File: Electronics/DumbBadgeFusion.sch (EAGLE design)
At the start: 103 parts, among them IC1 SN74CBT16233DGGR, IC2 SN74CBT16233DGGR, SW1 SPST_TACT-KMR2, U1 TDP3E001DRLR-SOT-23-5SOT-23-5, U6 MAX3232, U7 TPS61090RSAR, U8 MCP73831T-2ACI/OT, X4 32.768

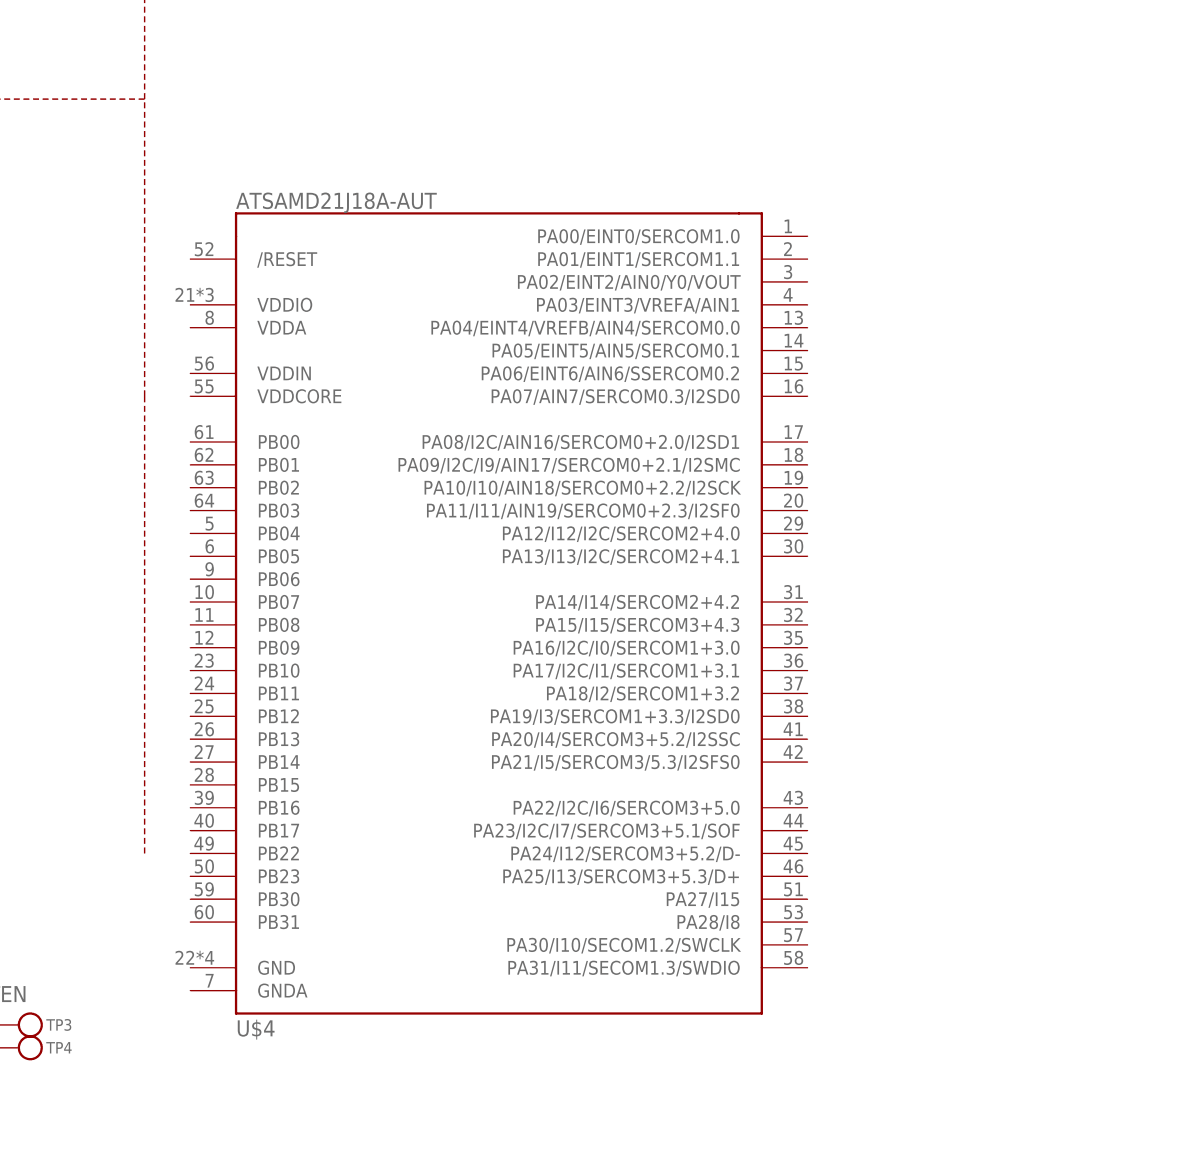
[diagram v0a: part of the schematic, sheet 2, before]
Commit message: beginning Firmware
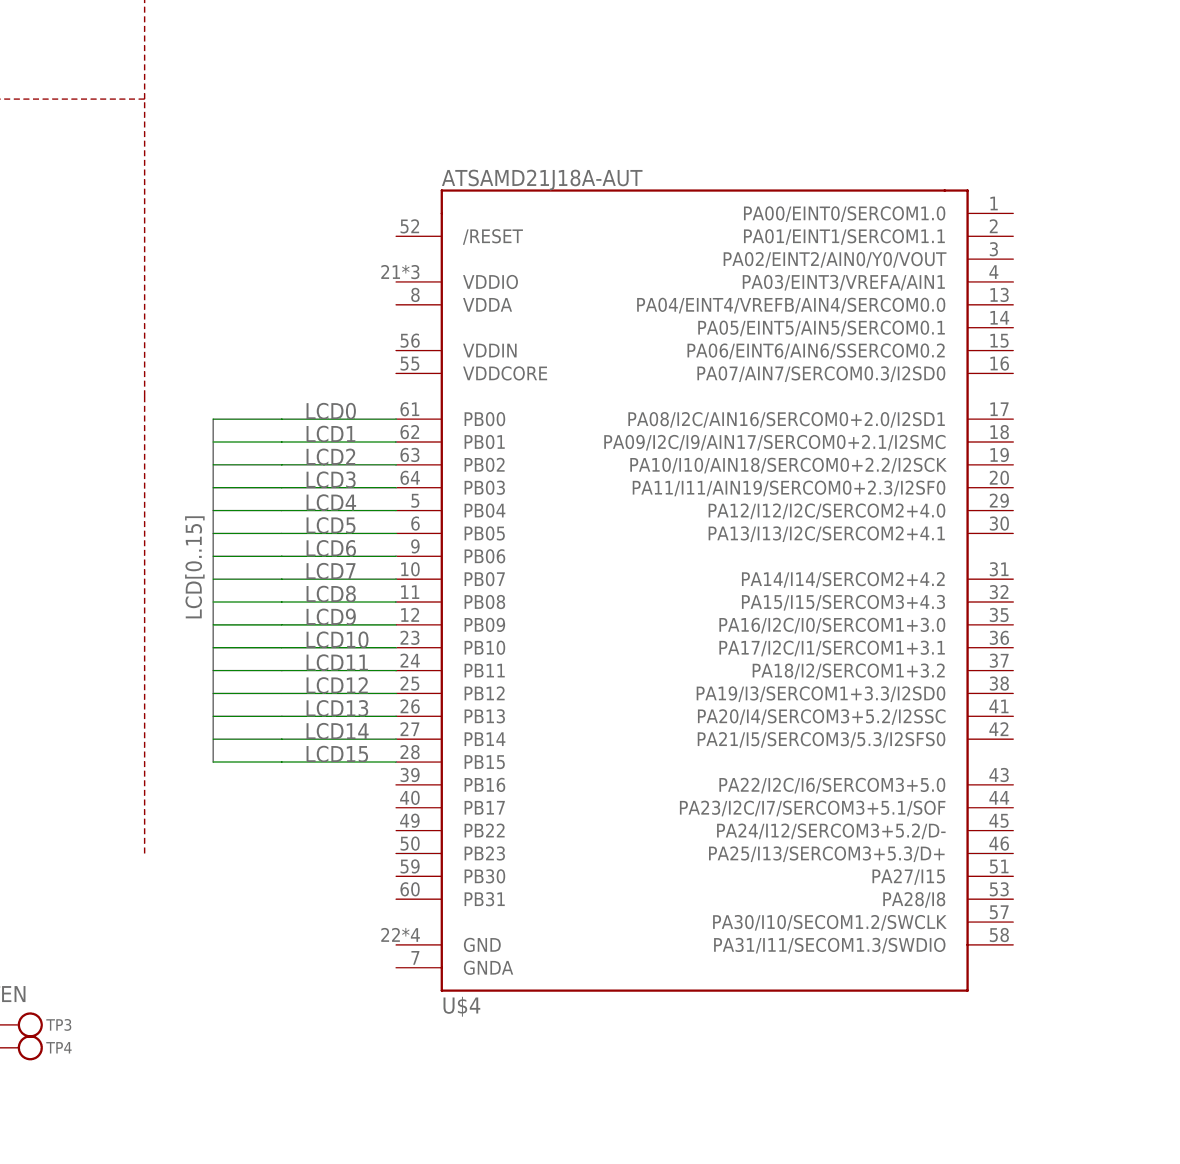
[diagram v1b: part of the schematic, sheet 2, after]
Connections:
- new net LCD0: U$4.PB00
- new net LCD1: U$4.PB01
- new net LCD10: U$4.PB10
- new net LCD11: U$4.PB11
- new net LCD12: U$4.PB12
- new net LCD13: U$4.PB13
- new net LCD14: U$4.PB14
- new net LCD15: U$4.PB15
- new net LCD2: U$4.PB02
- new net LCD3: U$4.PB03
- new net LCD4: U$4.PB04
- new net LCD5: U$4.PB05
- new net LCD6: U$4.PB06
- new net LCD7: U$4.PB07
- new net LCD8: U$4.PB08
- new net LCD9: U$4.PB09
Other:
- moved on the sheet: U$4
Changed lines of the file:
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@@
 <attribute name="SHEET" x="363.22" y="-0.635" size="2.54" layer="94" font="vector"/>
 </instance>
-<instance part="U$4" gate="G$1" x="152.4" y="78.74" smashed="yes">
-<attribute name="NAME" x="137.16" y="12.7" size="1.778" layer="95"/>
-<attribute name="VALUE" x="137.16" y="104.648" size="1.778" layer="96"/>
+<instance part="U$4" gate="G$1" x="175.26" y="81.28" smashed="yes">
+<attribute name="NAME" x="160.02" y="15.24" size="1.778" layer="95"/>
+<attribute name="VALUE" x="160.02" y="107.188" size="1.778" layer="96"/>
 </instance>
 <instance part="IC1" gate="G$1" x="248.92" y="226.06" smashed="yes">
@@
 </instances>
 <busses>
+<bus name="LCD[0..15]">
+<segment>
+<wire x1="134.62" y1="81.28" x2="134.62" y2="43.18" width="0.762" layer="92"/>
+<label x="133.35" y="58.928" size="1.778" layer="95" rot="R90"/>
+</segment>
+</bus>
 </busses>
 <nets>
@@
 </segment>
 </net>
+<net name="LCD0" class="0">
+<segment>
+<wire x1="134.62" y1="81.28" x2="142.24" y2="81.28" width="0.1524" layer="91"/>
+<wire x1="142.24" y1="81.28" x2="154.94" y2="81.28" width="0.1524" layer="91"/>
+<label x="144.78" y="81.28" size="1.778" layer="95"/>
+<pinref part="U$4" gate="G$1" pin="PB00"/>
+</segment>
+</net>
+<net name="LCD1" class="0">
+<segment>
+<wire x1="134.62" y1="78.74" x2="142.24" y2="78.74" width="0.1524" layer="91"/>
+<wire x1="142.24" y1="78.74" x2="154.94" y2="78.74" width="0.1524" layer="91"/>
+<label x="144.78" y="78.74" size="1.778" layer="95"/>
+<pinref part="U$4" gate="G$1" pin="PB01"/>
+</segment>
+</net>
+<net name="LCD2" class="0">
+<segment>
+<wire x1="134.62" y1="76.2" x2="142.24" y2="76.2" width="0.1524" layer="91"/>
+<wire x1="142.24" y1="76.2" x2="154.94" y2="76.2" width="0.1524" layer="91"/>
+<label x="144.78" y="76.2" size="1.778" layer="95"/>
+<pinref part="U$4" gate="G$1" pin="PB02"/>
+</segment>
+</net>
+<net name="LCD3" class="0">
+<segment>
+<wire x1="134.62" y1="73.66" x2="142.24" y2="73.66" width="0.1524" layer="91"/>
+<wire x1="142.24" y1="73.66" x2="154.94" y2="73.66" width="0.1524" layer="91"/>
+<label x="144.78" y="73.66" size="1.778" layer="95"/>
+<pinref part="U$4" gate="G$1" pin="PB03"/>
+</segment>
+</net>
+<net name="LCD4" class="0">
+<segment>
+<wire x1="134.62" y1="71.12" x2="142.24" y2="71.12" width="0.1524" layer="91"/>
+<wire x1="142.24" y1="71.12" x2="154.94" y2="71.12" width="0.1524" layer="91"/>
+<label x="144.78" y="71.12" size="1.778" layer="95"/>
+<pinref part="U$4" gate="G$1" pin="PB04"/>
+</segment>
+</net>
+<net name="LCD5" class="0">
+<segment>
+<wire x1="134.62" y1="68.58" x2="142.24" y2="68.58" width="0.1524" layer="91"/>
+<wire x1="142.24" y1="68.58" x2="154.94" y2="68.58" width="0.1524" layer="91"/>
+<label x="144.78" y="68.58" size="1.778" layer="95"/>
+<pinref part="U$4" gate="G$1" pin="PB05"/>
+</segment>
+</net>
+<net name="LCD6" class="0">
+<segment>
+<wire x1="134.62" y1="66.04" x2="142.24" y2="66.04" width="0.1524" layer="91"/>
+<wire x1="142.24" y1="66.04" x2="154.94" y2="66.04" width="0.1524" layer="91"/>
+<label x="144.78" y="66.04" size="1.778" layer="95"/>
+<pinref part="U$4" gate="G$1" pin="PB06"/>
+</segment>
+</net>
+<net name="LCD7" class="0">
+<segment>
+<wire x1="134.62" y1="63.5" x2="142.24" y2="63.5" width="0.1524" layer="91"/>
+<wire x1="142.24" y1="63.5" x2="154.94" y2="63.5" width="0.1524" layer="91"/>
+<label x="144.78" y="63.5" size="1.778" layer="95"/>
+<pinref part="U$4" gate="G$1" pin="PB07"/>
+</segment>
+</net>
+<net name="LCD8" class="0">
+<segment>
+<wire x1="134.62" y1="60.96" x2="142.24" y2="60.96" width="0.1524" layer="91"/>
+<wire x1="142.24" y1="60.96" x2="154.94" y2="60.96" width="0.1524" layer="91"/>
+<label x="144.78" y="60.96" size="1.778" layer="95"/>
+<pinref part="U$4" gate="G$1" pin="PB08"/>
+</segment>
+</net>
+<net name="LCD9" class="0">
+<segment>
+<wire x1="134.62" y1="58.42" x2="142.24" y2="58.42" width="0.1524" layer="91"/>
+<wire x1="142.24" y1="58.42" x2="154.94" y2="58.42" width="0.1524" layer="91"/>
+<label x="144.78" y="58.42" size="1.778" layer="95"/>
+<pinref part="U$4" gate="G$1" pin="PB09"/>
+</segment>
+</net>
+<net name="LCD10" class="0">
+<segment>
+<wire x1="134.62" y1="55.88" x2="142.24" y2="55.88" width="0.1524" layer="91"/>
+<wire x1="142.24" y1="55.88" x2="154.94" y2="55.88" width="0.1524" layer="91"/>
+<label x="144.78" y="55.88" size="1.778" layer="95"/>
+<pinref part="U$4" gate="G$1" pin="PB10"/>
+</segment>
+</net>
+<net name="LCD11" class="0">
+<segment>
+<wire x1="134.62" y1="53.34" x2="142.24" y2="53.34" width="0.1524" layer="91"/>
+<wire x1="142.24" y1="53.34" x2="154.94" y2="53.34" width="0.1524" layer="91"/>
+<label x="144.78" y="53.34" size="1.778" layer="95"/>
+<pinref part="U$4" gate="G$1" pin="PB11"/>
+</segment>
+</net>
+<net name="LCD12" class="0">
+<segment>
+<wire x1="134.62" y1="50.8" x2="142.24" y2="50.8" width="0.1524" layer="91"/>
+<wire x1="142.24" y1="50.8" x2="154.94" y2="50.8" width="0.1524" layer="91"/>
+<label x="144.78" y="50.8" size="1.778" layer="95"/>
+<pinref part="U$4" gate="G$1" pin="PB12"/>
+</segment>
+</net>
+<net name="LCD13" class="0">
+<segment>
+<wire x1="134.62" y1="48.26" x2="142.24" y2="48.26" width="0.1524" layer="91"/>
+<wire x1="142.24" y1="48.26" x2="154.94" y2="48.26" width="0.1524" layer="91"/>
+<label x="144.78" y="48.26" size="1.778" layer="95"/>
+<pinref part="U$4" gate="G$1" pin="PB13"/>
+</segment>
+</net>
+<net name="LCD14" class="0">
+<segment>
+<wire x1="134.62" y1="45.72" x2="142.24" y2="45.72" width="0.1524" layer="91"/>
+<wire x1="142.24" y1="45.72" x2="154.94" y2="45.72" width="0.1524" layer="91"/>
+<label x="144.78" y="45.72" size="1.778" layer="95"/>
+<pinref part="U$4" gate="G$1" pin="PB14"/>
+</segment>
+</net>
+<net name="LCD15" class="0">
+<segment>
+<wire x1="134.62" y1="43.18" x2="142.24" y2="43.18" width="0.1524" layer="91"/>
+<wire x1="142.24" y1="43.18" x2="154.94" y2="43.18" width="0.1524" layer="91"/>
+<label x="144.78" y="43.18" size="1.778" layer="95"/>
+<pinref part="U$4" gate="G$1" pin="PB15"/>
+</segment>
+</net>
